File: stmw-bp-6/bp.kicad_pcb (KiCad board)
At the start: 2 copper layers, 100 x 67 mm, 8 parts, among them J1 Conn_02x25_Odd_Even, J2 Conn_02x25_Odd_Even, U1 X1611WVS-98-9TV01, U2 X1611WVS-98-9TV01, U3 X1611WVS-98-9TV01, U4 X1611WVS-98-9TV01, U5 X1611WVS-98-9TV01, U6 X1611WVS-98-9TV01

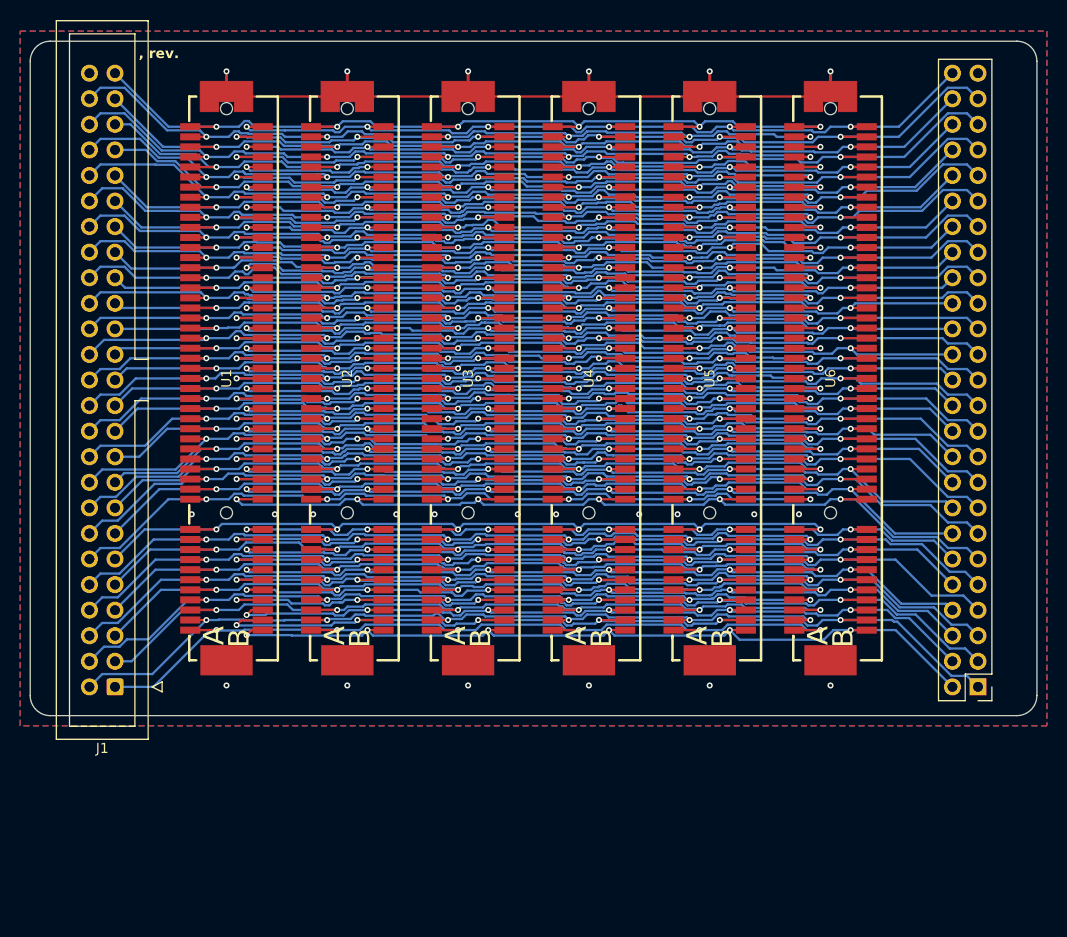
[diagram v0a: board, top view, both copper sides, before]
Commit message: Changes
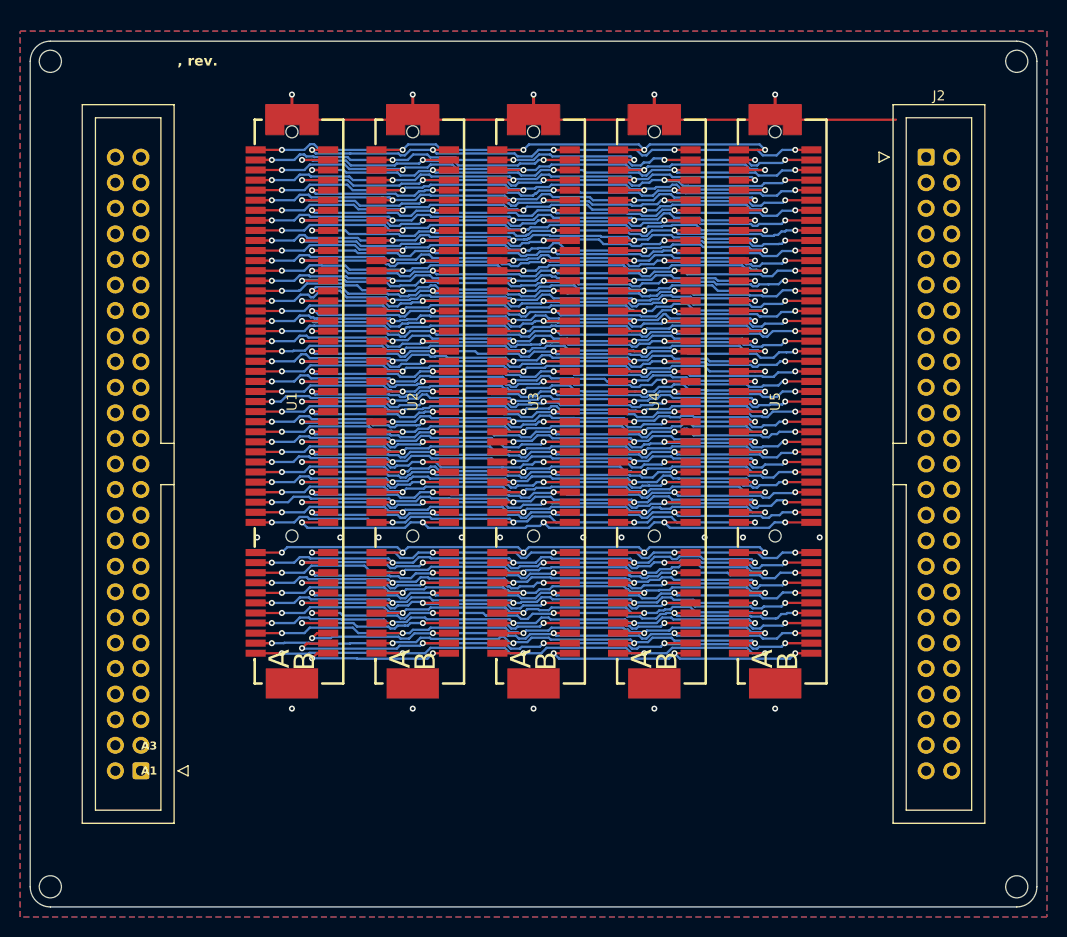
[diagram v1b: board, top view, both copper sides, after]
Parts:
- removed U6: X1611WVS-98-9TV01, stm32world:CONN-SMD_98P-P1.00-V_3133
- added H1: MountingHole, MountingHole:MountingHole_2.2mm_M2_DIN965, F.Cu at (92.0, 124.0)
- added H2: MountingHole, MountingHole:MountingHole_2.2mm_M2_DIN965, F.Cu at (188.0, 124.0)
- added H3: MountingHole, MountingHole:MountingHole_2.2mm_M2_DIN965, F.Cu at (188.0, 42.0)
- added H4: MountingHole, MountingHole:MountingHole_2.2mm_M2_DIN965, F.Cu at (92.0, 42.0)
- J2: footprint Connector_PinHeader_2.54mm:PinHeader_2x25_P2.54mm_Vertical -> Connector_IDC:IDC-Header_2x25_P2.54mm_Vertical
- moved J2 52.9 mm to (179.0, 51.5), turned to 0 degrees
- moved J1 8.73 mm to (101.0, 112.5)
- moved U1 6.89 mm to (116.0, 75.8)
- moved U2 6.89 mm to (128.0, 75.8)
- moved U3 6.89 mm to (140.0, 75.8)
- moved U4 6.89 mm to (152.0, 75.8)
- moved U5 6.89 mm to (164.0, 75.8)
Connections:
- J2 pad 1: B2 -> GND
- J2 pad 10: B9 -> B41
- J2 pad 11: B12 -> B40
- J2 pad 12: B11 -> B39
- J2 pad 13: B14 -> B38
- J2 pad 14: B13 -> B37
- J2 pad 15: B16 -> B36
- J2 pad 16: B15 -> B35
- J2 pad 17: B18 -> B34
- J2 pad 18: B17 -> B33
- J2 pad 19: B20 -> B32
- J2 pad 2: B1 -> B49
- J2 pad 20: B19 -> B31
- J2 pad 21: B22 -> B30
- J2 pad 22: B21 -> B29
- J2 pad 23: B24 -> B28
- J2 pad 24: B23 -> B27
- J2 pad 27: B28 -> B24
- J2 pad 28: B27 -> B23
- J2 pad 29: B30 -> B22
- J2 pad 3: B4 -> B48
- J2 pad 30: B29 -> B21
- J2 pad 31: B32 -> B20
- J2 pad 32: B31 -> B19
- J2 pad 33: B34 -> B18
- J2 pad 34: B33 -> B17
- J2 pad 35: B36 -> B16
- J2 pad 36: B35 -> B15
- J2 pad 37: B38 -> B14
- J2 pad 38: B37 -> B13
- J2 pad 39: B40 -> B12
- J2 pad 4: B3 -> B47
- J2 pad 40: B39 -> B11
- J2 pad 41: B42 -> B10
- J2 pad 42: B41 -> B9
- J2 pad 43: B44 -> B8
- J2 pad 44: B43 -> B7
- J2 pad 45: B46 -> B6
- J2 pad 46: B45 -> B5
- J2 pad 47: B48 -> B4
- J2 pad 48: B47 -> B3
- J2 pad 49: GND -> B2
- J2 pad 5: B6 -> B46
- J2 pad 50: B49 -> B1
- J2 pad 6: B5 -> B45
- J2 pad 7: B8 -> B44
- J2 pad 8: B7 -> B43
- J2 pad 9: B10 -> B42
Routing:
- net A48: track 85.8 -> 45.3 mm, vias 6 -> 5
- net B1: track 84.6 -> 45.3 mm, vias 6 -> 5
- net B2: track 94.2 -> 62.7 mm, vias 6 -> 5
- net B4: track 94.0 -> 62.8 mm, vias 6 -> 5
- net B48: track 94.1 -> 62.9 mm, vias 6 -> 5
- net B12: track 94.0 -> 62.8 mm, vias 6 -> 5
- net B6: track 93.9 -> 62.9 mm, vias 6 -> 5
- net B14: track 93.9 -> 63.0 mm, vias 6 -> 5
- net B46: track 93.8 -> 62.8 mm, vias 6 -> 5
- net B8: track 93.6 -> 62.8 mm, vias 6 -> 5
- net B44: track 93.5 -> 62.8 mm, vias 6 -> 5
- net B16: track 93.5 -> 62.8 mm, vias 6 -> 5
- net B10: track 93.7 -> 63.1 mm, vias 6 -> 5
- net B42: track 93.3 -> 62.8 mm, vias 6 -> 5
- net B18: track 93.3 -> 62.8 mm, vias 6 -> 5
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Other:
- board size 100 x 67 mm -> 100 x 86 mm
- board text added: "A1"
- board text added: "A3"
